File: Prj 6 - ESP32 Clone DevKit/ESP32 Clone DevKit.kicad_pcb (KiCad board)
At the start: 4 copper layers, 0 parts

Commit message: Trying to do differential tracks
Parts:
- added C1: 22nF/10V(20%), Capacitor_SMD:C_0201_0603Metric, B.Cu at (125.3, 93.1)
- added C14: 0.1uF/50V(10%), Capacitor_SMD:C_01005_0402Metric, F.Cu at (120.9, 91.3)
- added C15: 0.1uF/50V(10%)(NC), Capacitor_SMD:C_01005_0402Metric, F.Cu at (136.2, 91.3)
- added C19: 0.1uF/50V(10%), Capacitor_SMD:C_01005_0402Metric, F.Cu at (130.1, 91.3)
- added C20: 4.7uF/6.3V(10%), Capacitor_SMD:C_01005_0402Metric, F.Cu at (127.0, 91.3)
- added C21: 22u/10V(20%), Capacitor_SMD:C_0201_0603Metric, F.Cu at (139.3, 91.3)
- added C22: 0.1u/50V(10%), Capacitor_SMD:C_01005_0402Metric, F.Cu at (123.9, 91.3)
- added C3: 22nF/10V(20%), Capacitor_SMD:C_0201_0603Metric, B.Cu at (135.8, 93.1)
- added C9: 0.1u/50V(10%), Capacitor_SMD:C_01005_0402Metric, F.Cu at (133.1, 91.3)
- added D1: RED LED, LED_SMD:LED_0603_1608Metric, F.Cu at (129.8, 85.5)
- added D3: BAT760-7, Diode_SMD:D_SOD-323, F.Cu at (138.2, 85.5)
- added D4: LESD5D5.0CT1G, Diode_SMD:D_SOD-523, F.Cu at (125.7, 85.5)
- added D5: LESD5D5.0CT1G, Diode_SMD:D_SOD-523, F.Cu at (134.0, 85.5)
- added D6: LESD5D5.0CT1G, Diode_SMD:D_SOD-523, F.Cu at (121.9, 85.5)
- added J1: USB CON8, #download:USB_Micro-AB_Molex_47590-0001, F.Cu at (130.5, 109.3)
- added J2: Conn_01x19_Pin, Connector_PinHeader_2.54mm:PinHeader_1x19_P2.54mm_Vertical, F.Cu at (117.0, 64.2)
- added J3: Conn_01x19_Pin, Connector_PinHeader_2.54mm:PinHeader_1x19_P2.54mm_Vertical, F.Cu at (144.0, 64.2)
- added Q1: MMSS8050-H-TP, #download:TRANS_MMSS8050-H-TP, F.Cu at (122.1, 108.4)
- added Q2: MMSS8050-H-TP, #download:TRANS_MMSS8050-H-TP, F.Cu at (138.9, 108.4)
- added R11: 10K(5%), Resistor_SMD:R_01005_0402Metric_Pad0.57x0.30mm_HandSolder, F.Cu at (123.9, 88.5)
- added R17: 0R(5%), Resistor_SMD:R_01005_0402Metric_Pad0.57x0.30mm_HandSolder, F.Cu at (136.4, 88.5)
- added R18: 0R(5%), Resistor_SMD:R_01005_0402Metric_Pad0.57x0.30mm_HandSolder, F.Cu at (138.9, 88.5)
- added R2: 2K(5%), Resistor_SMD:R_01005_0402Metric_Pad0.57x0.30mm_HandSolder, F.Cu at (126.4, 88.5)
- added R21: 10K(5%), Resistor_SMD:R_01005_0402Metric_Pad0.57x0.30mm_HandSolder, F.Cu at (122.1, 110.9)
- added R22: 10K(5%), Resistor_SMD:R_01005_0402Metric_Pad0.57x0.30mm_HandSolder, F.Cu at (138.9, 110.9)
- added R23: 10K(5%)(NC), Resistor_SMD:R_01005_0402Metric_Pad0.57x0.30mm_HandSolder, F.Cu at (121.4, 88.5)
- added R24: 2K(5%), Resistor_SMD:R_01005_0402Metric_Pad0.57x0.30mm_HandSolder, F.Cu at (128.9, 88.5)
- added R25: 22.1K(5%), Resistor_SMD:R_01005_0402Metric_Pad0.57x0.30mm_HandSolder, F.Cu at (131.4, 88.5)
- added R26: 47.5K(5%), Resistor_SMD:R_01005_0402Metric_Pad0.57x0.30mm_HandSolder, F.Cu at (133.9, 88.5)
- added SW1: SW_Push, #download:SW_SPST_B3S-1000, F.Cu at (136.0, 101.0)
- added SW2: SW_Push, #download:SW_SPST_B3S-1000, F.Cu at (125.0, 101.0)
- added U1: CP2102N-A01-GQFN28, Package_DFN_QFN:QFN-28-1EP_5x5mm_P0.5mm_EP3.35x3.35mm, B.Cu at (130.5, 97.2)
- added U2: AMS1117-3.3, Package_TO_SOT_SMD:SOT-223-3_TabPin2, B.Cu at (130.5, 87.0)
- added U3: ESP32-WROOM-32D, #download:MODULE_ESP32-WROOM-32D, F.Cu at (130.5, 68.2)
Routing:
- net VDD33: track 0.00 -> 73.6 mm, vias 0 -> 6
- net GND: track 0.00 -> 69.9 mm, vias 0 -> 39
- net /EN: track 0.00 -> 58.9 mm, vias 0 -> 4
- net VBUS: track 0.00 -> 57.3 mm
- net /IO0: track 0.00 -> 49.0 mm, vias 0 -> 3
- net EXT_5V: track 0.00 -> 42.4 mm, vias 0 -> 4
- net /DTR: track 0.00 -> 40.2 mm, vias 0 -> 1
- net /CLK: track 0.00 -> 38.4 mm
- net /RTS: track 0.00 -> 37.4 mm, vias 0 -> 3
- net /CMD: track 0.00 -> 36.4 mm
- net /SD0: track 0.00 -> 34.7 mm
- net /SD3: track 0.00 -> 32.8 mm
- net /SD1: track 0.00 -> 31.1 mm
- net /SD2: track 0.00 -> 29.1 mm
- net /TXD0: track 0.00 -> 29.0 mm, vias 0 -> 1
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- added copper zone on B.Cu, net GND
- added copper zone on In1.Cu, net GND
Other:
- board outline added: 31.1 x 56.8 mm
- board text added: "+"

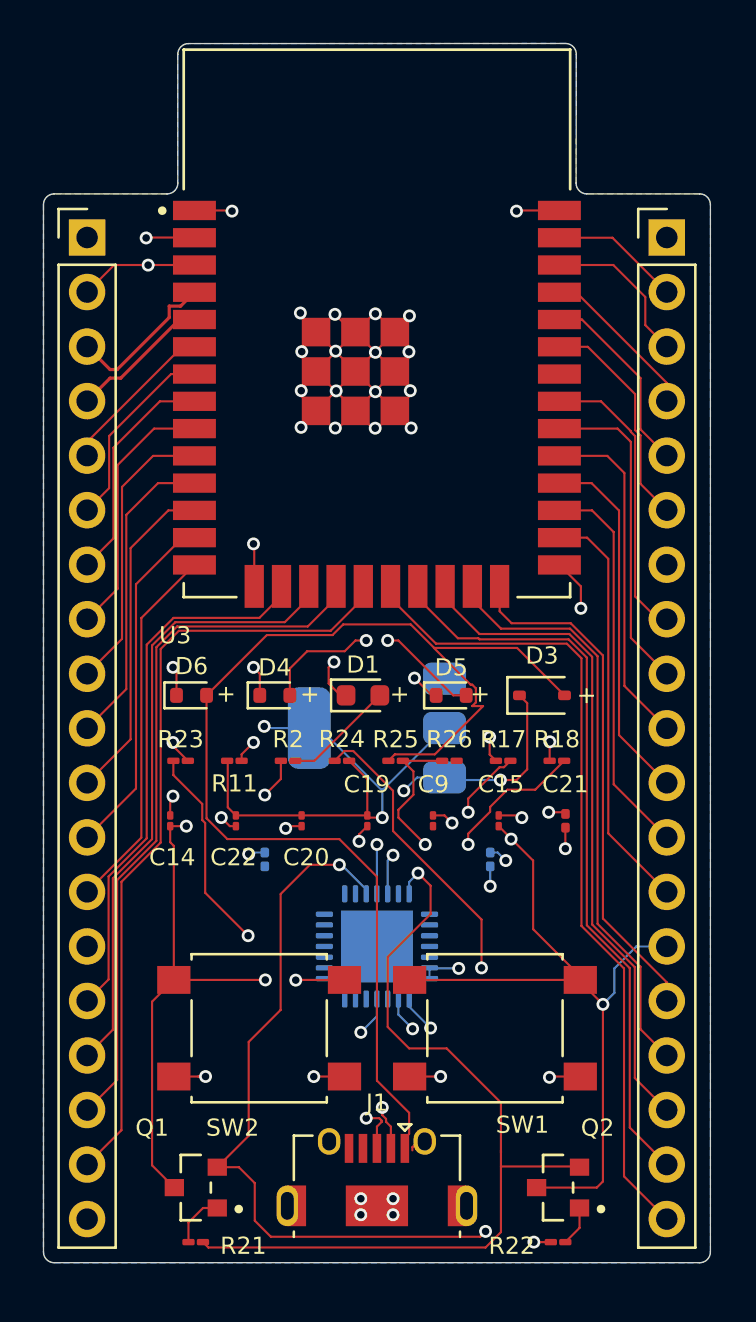
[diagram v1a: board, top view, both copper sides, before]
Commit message: Completed routing v0.1
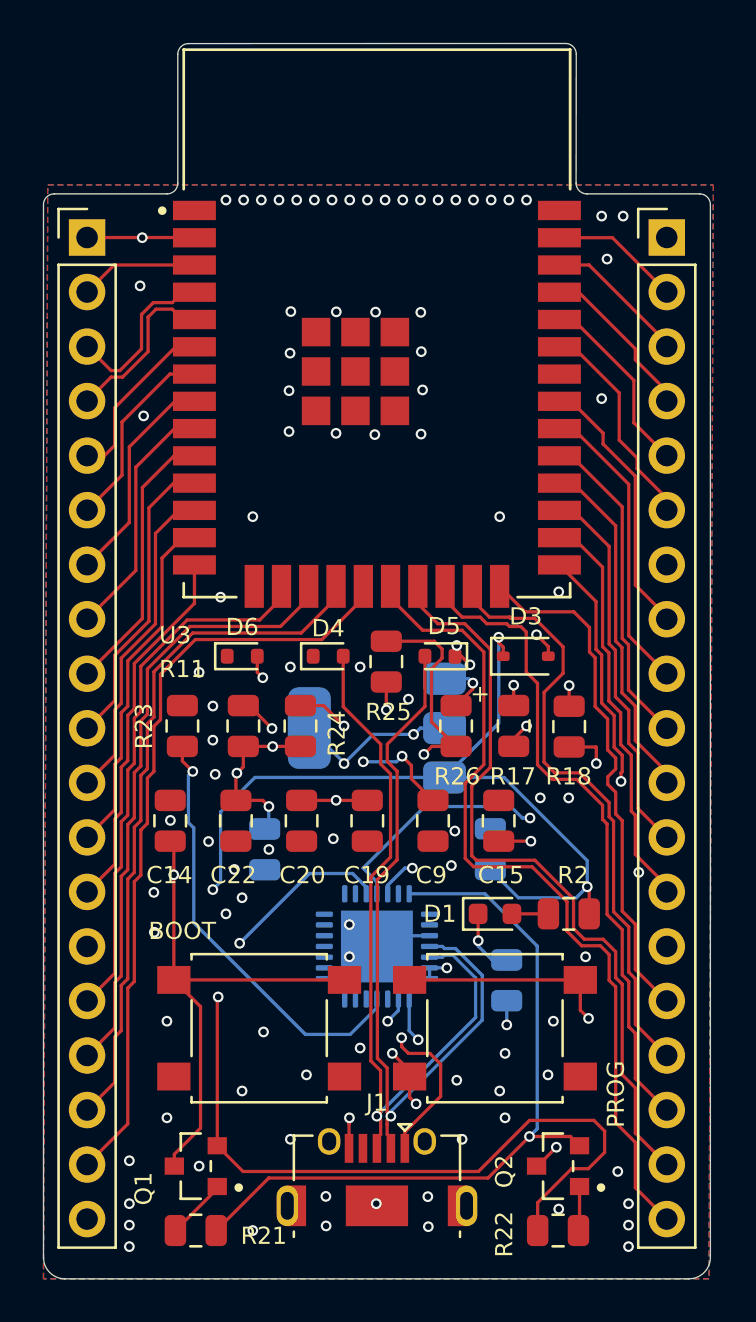
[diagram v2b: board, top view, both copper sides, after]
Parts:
- C1, C3: footprint Capacitor_SMD:C_0201_0603Metric -> Capacitor_SMD:C_0805_2012Metric
- C14, C15, C19, C20, C22, C9: footprint Capacitor_SMD:C_01005_0402Metric -> Capacitor_SMD:C_0805_2012Metric
- C21: footprint Capacitor_SMD:C_0201_0603Metric -> Capacitor_SMD:C_0805_2012Metric; moved to B.Cu
- R11, R17, R18, R2, R21, R22, R23, R24, R25, R26: footprint Resistor_SMD:R_01005_0402Metric_Pad0.57x0.30mm_HandSolder -> Capacitor_SMD:C_0805_2012Metric
- moved R2 14.9 mm to (139.4, 95.7), turned to 180 degrees
- moved D1 11.9 mm to (136.0, 95.7)
- moved C1 10.5 mm to (135.8, 92.6), turned to 90 degrees
- moved C3 10.5 mm to (125.3, 92.7), turned to -90 degrees
- moved C21 7.92 mm to (136.5, 98.7)
- moved R25 4.64 mm to (130.9, 83.9), turned to 90 degrees
- moved D4 3.08 mm to (128.2, 83.7)
- moved D6 2.98 mm to (124.2, 83.7)
- moved R24 2.52 mm to (126.9, 86.9), turned to 90 degrees
- moved D3 1.97 mm to (137.4, 83.7)
- moved D5 1.90 mm to (133.4, 83.7), turned to 180 degrees
- moved R17 1.70 mm to (136.9, 86.9), turned to -90 degrees
- moved R18 1.69 mm to (139.5, 86.9), turned to -90 degrees
- moved R11 1.67 mm to (124.3, 86.9), turned to 90 degrees
- moved R26 1.65 mm to (134.2, 86.9), turned to 90 degrees
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- renumbered SW2 to BOOT, SW1 to PROG
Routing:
- net GND: track 69.9 -> 18.4 mm, vias 39 -> 101
- net VDD33: track 73.6 -> 26.3 mm, vias 6 -> 9
- net VBUS: track 57.3 -> 41.2 mm, vias 0 -> 4
- net /USB_DP: track 20.1 -> 36.0 mm, vias 2 -> 1
- net EXT_5V: track 42.4 -> 57.4 mm, vias 4 -> 3
- net /USB_DN: track 21.6 -> 35.6 mm, vias 2 -> 1
- net /RXD: track 11.1 -> 22.4 mm
- net /TXD: track 12.1 -> 19.0 mm
- net Net-(U1-VBUS): track 18.6 -> 25.2 mm
- net /RTS: track 37.4 -> 43.8 mm, vias 3 -> 2
- net /DTR: track 40.2 -> 34.9 mm
- net /TXD0: track 29.0 -> 24.8 mm
- net Net-(D1-A): track 5.20 -> 1.70 mm
- net /RXD0: track 25.5 -> 22.3 mm
- net Net-(U1-~{RST}): track 20.8 -> 18.9 mm
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- added copper zone on F.Cu, net GND
- added copper zone on In2.Cu, net GND
- added copper zone on In2.Cu, net VDD33
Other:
- board size 31.1 x 56.8 mm -> 31.1 x 57.5 mm
- board text added: "ToDo: 1. Differential lines do not have uninterrupted ground underneath due to vias 2. The USB connector is not outside of the edge nor it has a notch"
